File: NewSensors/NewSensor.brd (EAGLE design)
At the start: 14.6 x 22.1 mm, 5 parts, among them X2 CNY70

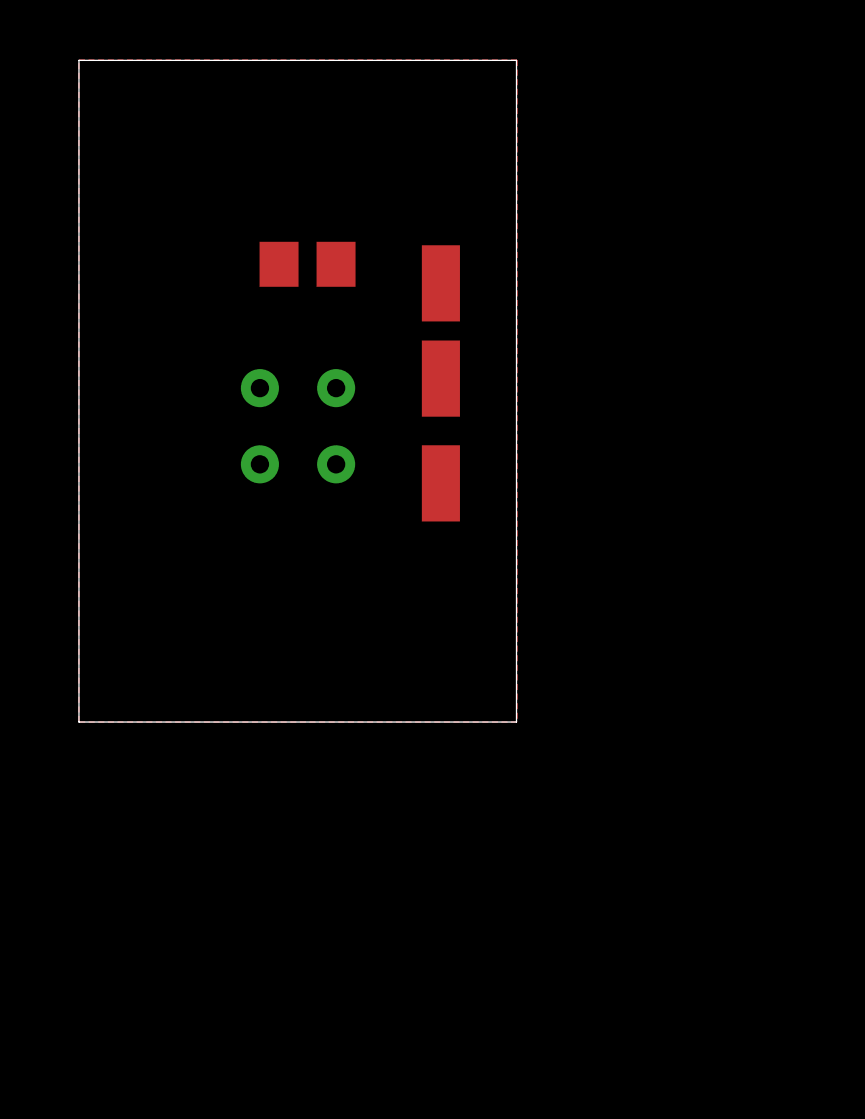
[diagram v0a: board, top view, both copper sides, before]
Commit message: Added code V1
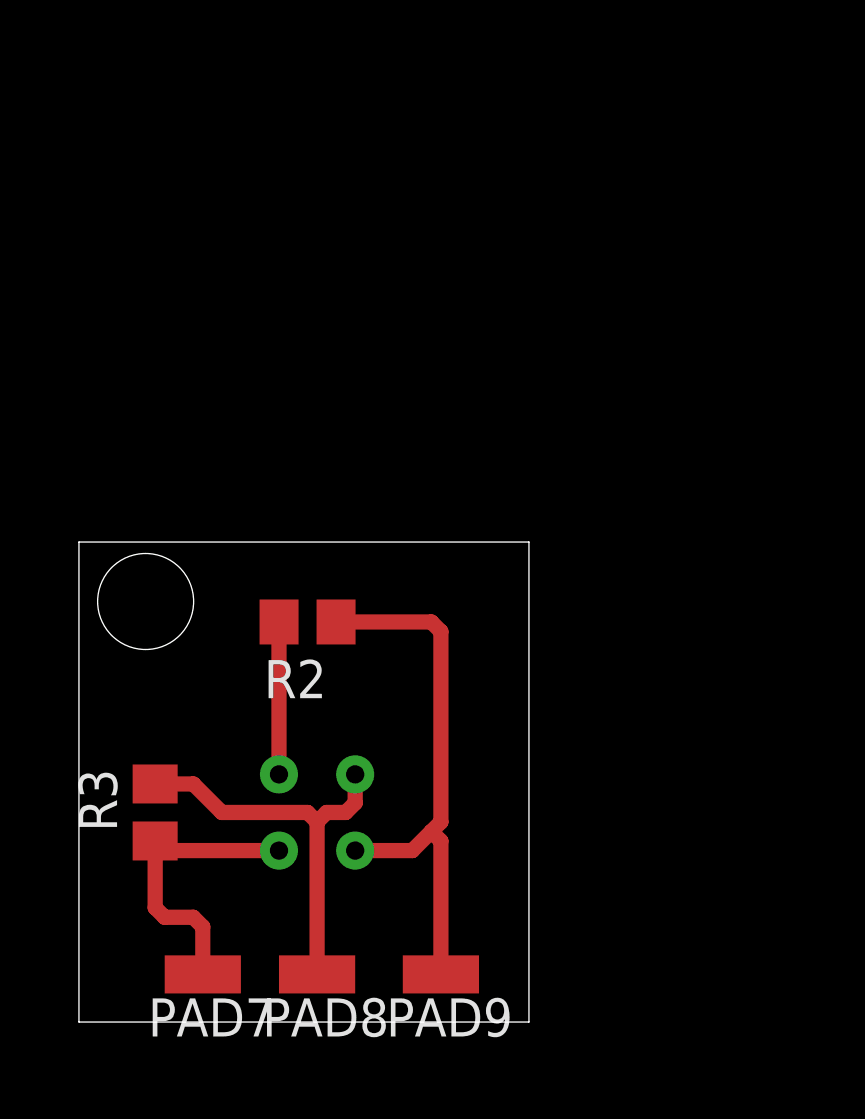
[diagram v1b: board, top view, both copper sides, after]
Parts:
- removed PAD4, PAD5, PAD6: WIREPADSMD1,27-254, wirepad:SMD1,27-2,54
- removed R1: (no value), ScyllAlarmV3.0:RCL_R0805
- removed X2: CNY70, cny70:4
- added PAD7, PAD8, PAD9: WIREPADSMD1,27-254, wirepad:SMD1,27-2,54
- added R2, R3: (no value), ScyllAlarmV3.0:RCL_R0805
- added X3: CNY70, cny70:4
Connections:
- removed net GND: PAD6.1, R1.1
- removed net N$1: R1.2, X2.K
- removed net SENSOR: PAD5.1, X2.E
- removed net VCC: PAD4.1, X2.A, X2.C
- new net GND_A: PAD9.1, R2.1, X3.E
- new net N$2: R2.2, X3.K
- new net SENSOR_A: PAD8.1, R3.2, X3.C
- new net VCC_A: PAD7.1, R3.1, X3.A
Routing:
- net GND_A: track 0.00 -> 18.1 mm
- net SENSOR_A: track 0.00 -> 13.5 mm
- net VCC_A: track 0.00 -> 9.92 mm
- net N$2: track 0.00 -> 5.08 mm
- removed copper zone on layer 1, net GND
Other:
- board size 14.6 x 22.1 mm -> 15 x 16 mm

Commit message: New sketch
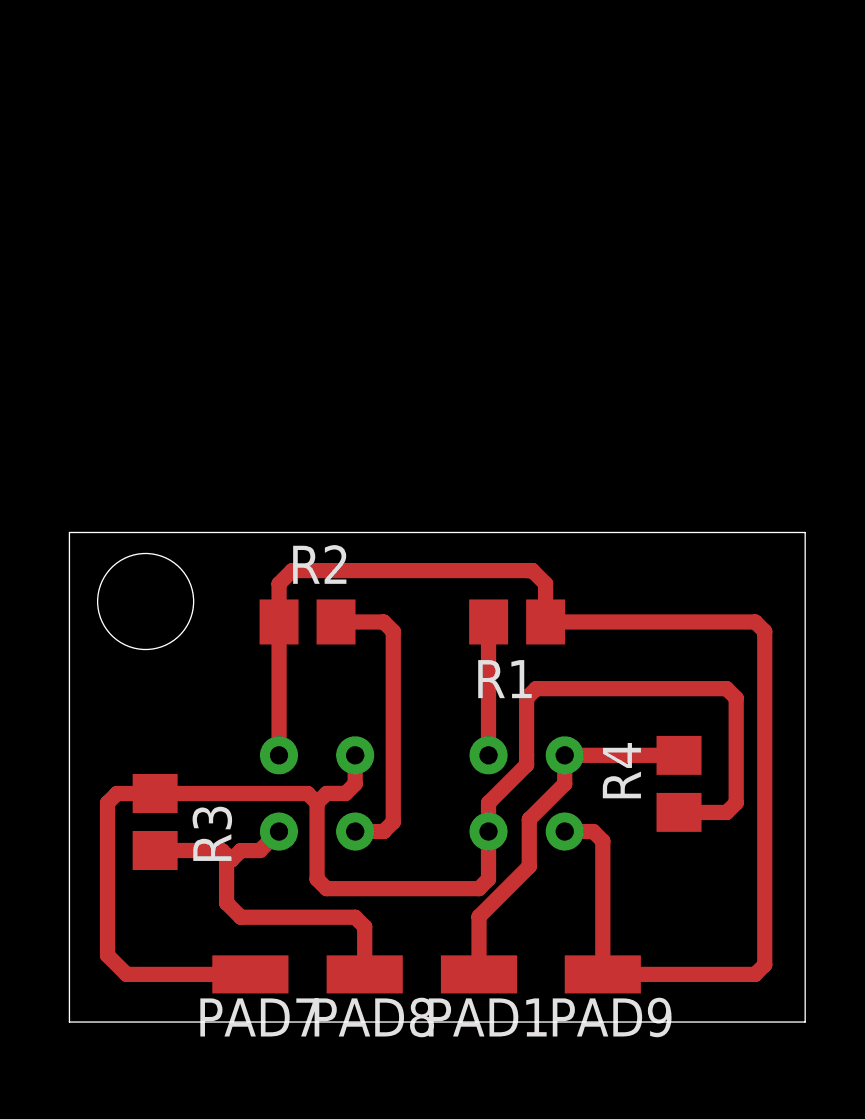
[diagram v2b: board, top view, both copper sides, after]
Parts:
- added PAD1: WIREPADSMD1,27-254, wirepad:SMD1,27-2,54
- added R1, R4: (no value), ScyllAlarmV3.0:RCL_R0805
- added X1: CNY70, cny70:4
- moved PAD9 5.40 mm to (17.5, 1.59)
- moved PAD8 1.59 mm to (9.53, 1.59)
- moved PAD7 1.59 mm to (5.71, 1.59)
- moved X3 0.63 mm to (7.94, 7.62), turned to 0 degrees
- moved R3 0.32 mm to (2.54, 6.67), turned to 270 degrees
- turned R2 to 0 degrees
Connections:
- new net N$1: R1.2, X1.K
- new net SENSOR_B: PAD1.1, R4.2, X1.C
- net GND_A: now also R1.1, X1.E
- net VCC_A: now also R4.1, X1.A
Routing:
- net VCC_A: track 9.92 -> 47.8 mm
- net GND_A: track 18.1 -> 46.4 mm
- net SENSOR_B: track 0.00 -> 12.3 mm
- net N$2: track 5.08 -> 9.79 mm
- net N$1: track 0.00 -> 4.45 mm
- net SENSOR_A: track 13.5 -> 12.8 mm
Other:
- board size 15 x 16 mm -> 24.5 x 16.3 mm
